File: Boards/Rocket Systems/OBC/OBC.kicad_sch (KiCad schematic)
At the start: 68 parts, among them IC1 NEO-M8Q-0, IC2 NSVT30010MXV6T1G, IC3 BC846BLT1G, J1 22027063, J2 5023520200, J3 SMARA_CONNECTOR, Q1 BC857CMB_315, U1 VLMKG3400-GS08, U2 LIS2MDLTR, U3 BMI323, U4 LSM6DSOTR, U5 LPS22DFTR, U6 BMP581

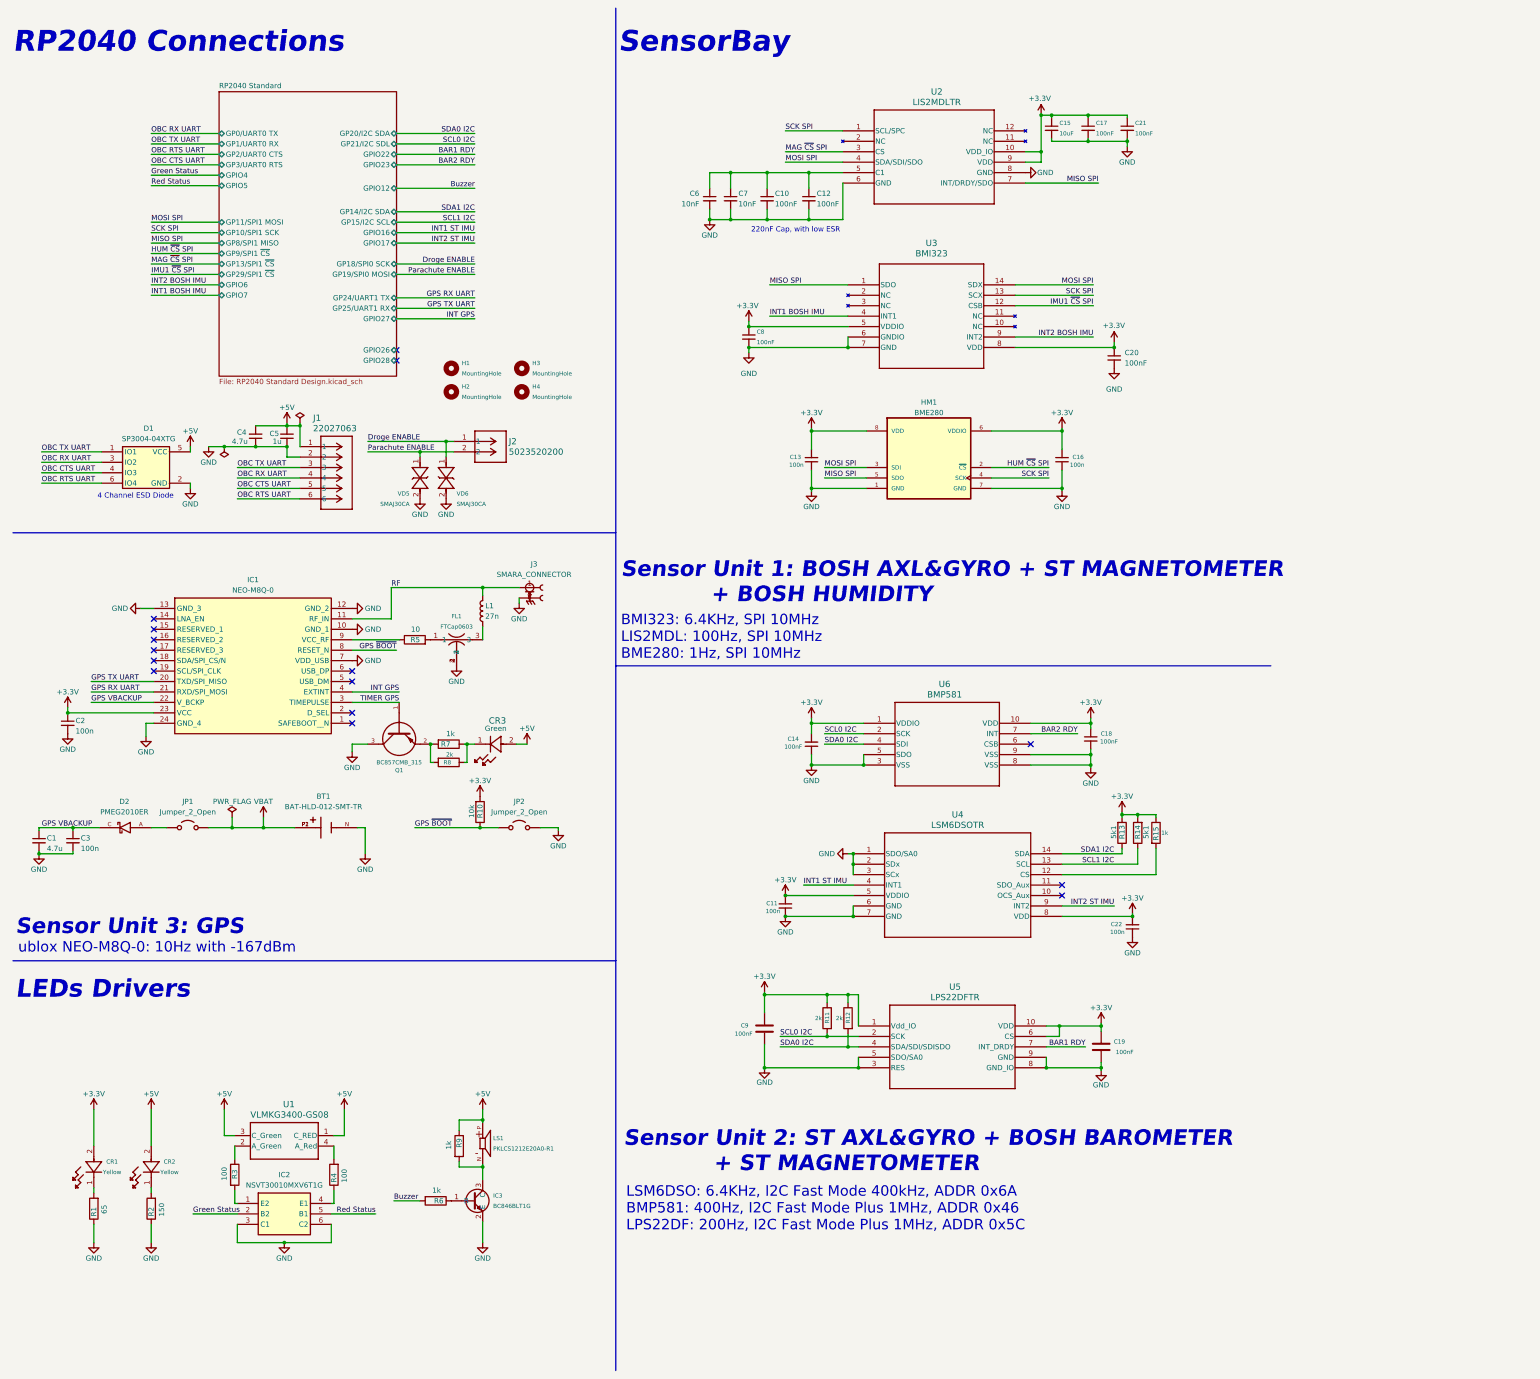
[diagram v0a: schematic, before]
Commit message: Repo rename and update
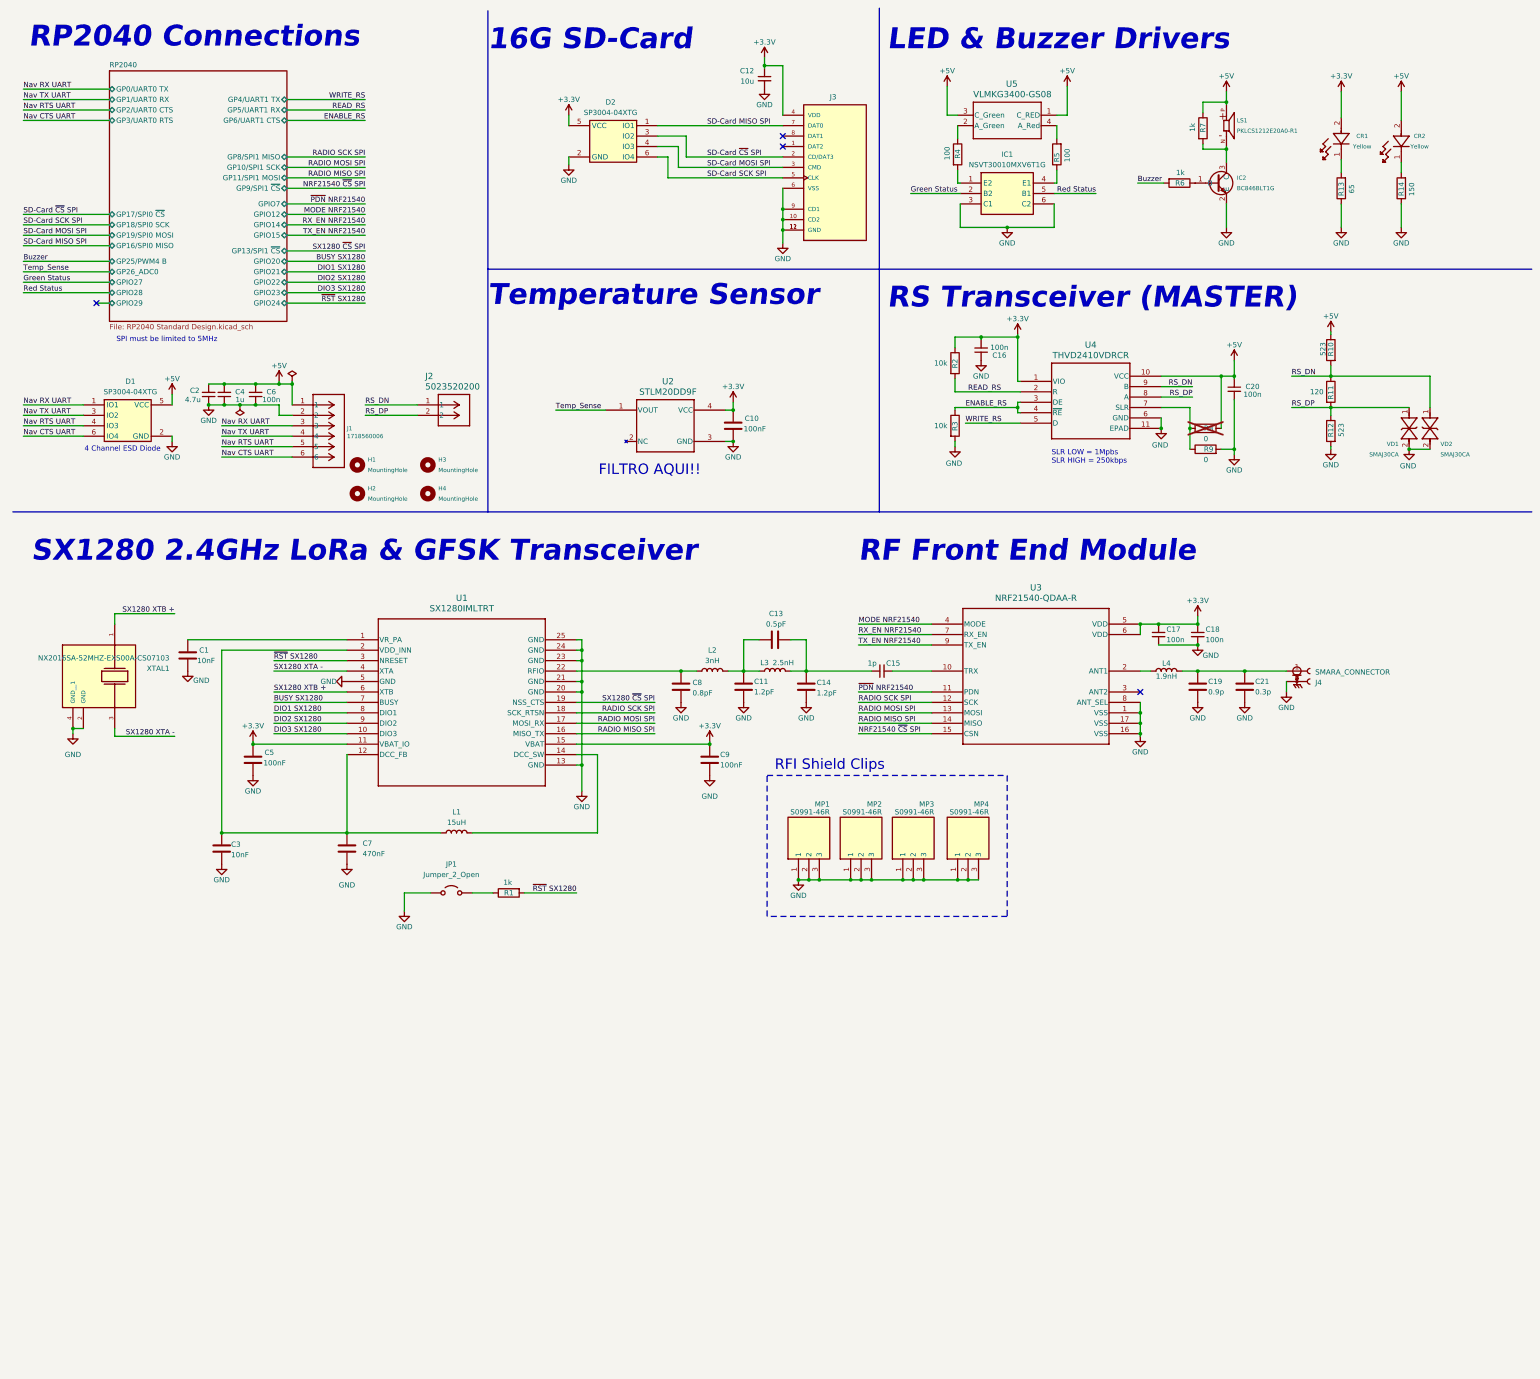
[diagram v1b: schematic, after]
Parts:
- removed BT1: BAT-HLD-012-SMT-TR, BAT_HLD_012:BAT_BAT-HLD-012-SMT-TR, symbol BAT-HLD-012-SMT-TR:BAT-HLD-012-SMT-TR
- removed C1: 4.7u, Capacitor-0402:Capacitor_0402, symbol Device:C_Small
- removed C10, C14, C21, C8: 100nF, Capacitor-0402:Capacitor_0402, symbol Device:C_Small
- removed C11, C13, C22, C3: 100n, Capacitor-0402:Capacitor_0402, symbol Device:C_Small
- removed C5: 1u, Capacitor-0402:Capacitor_0402, symbol Device:C_Small
- removed C7: 10nF, Capacitor-0402:Capacitor_0402, symbol Device:C_Small
- removed CR3: VLMC3100-GS08, LED-Green_VLMC3100-GS08:LED_PLCC_VSMB, symbol GreenLED__VLMC3100-GS08:VLMC3100-GS08
- removed D2: PMEG2010ER, Diode-Schottky_PMEG2010ER:SODFL3517X110N, symbol PMEG2010ER:PMEG2010ER
- removed FL1: FTCap0603, FTCap_0603:FTCap_0603, symbol FTCap0603:FTCap0603
- removed HM1: BME280, BME280:BME280, symbol BME280:BME280
- removed IC1: NEO-M8Q-0, NEO-M8Q-0:NEO-M8_UBL, symbol NEO-M8Q-0:NEO-M8Q-0
- removed IC2: NSVT30010MXV6T1G, 2 PNP:SOT-563_1P3X1P7_ONS, symbol NSVT30010MXV6T1G:NSVT30010MXV6T1G
- removed IC3: BC846BLT1G, BJT NPN:SOT96P237X111-3N, symbol BC846BLT1G:BC846BLT1G
- removed J1: 22027063, 6 Female Conn:CONN6X1_22027063_MOL, symbol 022027063:22027063
- removed J3: SMARA_CONNECTOR, Side Angle SMA:SMARACONNECTOR, symbol SMARA_CONNECTOR:SMARA_CONNECTOR
- removed JP2: Jumper_2_Open, Jumper:SolderJumper-2_P1.3mm_Open_RoundedPad1.0x1.5mm, symbol Jumper:Jumper_2_Open
- removed Q1: BC857CMB_315, PNP_BC857CMB_315:TRANS_PMZB550UNEYL, symbol BC857CMB_315:BC857CMB_315
- removed R15: 1k, Resistor-0402:RES_0402, symbol Device:R
- removed U1: VLMKG3400-GS08, VLMKG3400-GS08:SMT_00-GS08_VIS, symbol VLMKG3400-GS08:VLMKG3400-GS08
- removed U2: LIS2MDLTR, MAG LIS2MDLTR:LGA-12_2X2X1_STM, symbol MAG_LIS2MDLTR:LIS2MDLTR
- removed U3: BMI323, IMU BMI323:BMI323_BOS, symbol IMU_BMI323:BMI323
- removed U4: LSM6DSOTR, LSM6DSOTR:LGA-14L_2P5X3X0P86_STM, symbol LSM6DSOTR:LSM6DSOTR
- removed U5: LPS22DFTR, BARO LPS22DFTR:QFN_22DFTR_STM, symbol BARO_LPS22DFTR:LPS22DFTR
- removed U6: BMP581, BARO BMP581:QFN10_BMP581_BOS, symbol BARO_BMP581:BMP581
- removed VD5, VD6: SMAJ30CA, SMAJ30CA:SMASeries_LTF, symbol SMAJ30CA:SMAJ30CA
- added C1, C3: 10nF, Capacitor-0402:Capacitor_0402, symbol Device:C
- added C10, C5: 100nF, Capacitor-0402:Capacitor_0402, symbol Device:C
- added C11, C14: 1.2pF, Capacitor-0402:Capacitor_0402, symbol Device:C
- added C13: 0.5pF, Capacitor-0402:Capacitor_0402, symbol Device:C
- added C21: 0.3p, Capacitor-0402:Capacitor_0402, symbol Device:C
- added C7: 470nF, Capacitor-0402:Capacitor_0402, symbol Device:C
- added C8: 0.8pF, Capacitor-0402:Capacitor_0402, symbol Device:C
- added D2: SP3004-04XTG, TVS-SP3004:SOT563_LTF, symbol SP3004-04XTG:SP3004-04XTG
- added IC1: NSVT30010MXV6T1G, 2 PNP:SOT-563_1P3X1P7_ONS, symbol NSVT30010MXV6T1G:NSVT30010MXV6T1G
- added IC2: BC846BLT1G, BJT NPN:SOT96P237X111-3N, symbol BC846BLT1G:BC846BLT1G
- added J1: 1718560006, 6 Male Conn:CONN06_1718560006_MOL, symbol 1718560006:1718560006
- added J3: MEM2061-01-188-00-A_REVA, SD-CARD_MEM2061-01-188-00-A:GCT_MEM2061-01-188-00-A_REVA, symbol MEM2061-01-188-00-A_REVA:MEM2061-01-188-00-A_REVA
- added J4: SMARA_CONNECTOR, Side Angle SMA:SMARACONNECTOR, symbol SMARA_CONNECTOR:SMARA_CONNECTOR
- added L2: 3nH, Inductor-0402:Inductor_0402, symbol Device:L
- added L3: 2.5nH, Inductor-0402:Inductor_0402, symbol Device:L
- added L4: 1.9nH, Inductor-0201:Inductor_0201, symbol Device:L
- added MP1, MP2, MP3, MP4: S0991-46R, S0991-46R:S099146R, symbol S0991-46R:S0991-46R
- added U1: SX1280IMLTRT, SX1280:QFN24_4X4_SEM, symbol SX1280:SX1280IMLTRT
- added U2: STLM20DD9F, STLM20DD9F:UDFN-4L_STM, symbol STLM20DD9F:STLM20DD9F
- added U3: NRF21540-QDAA-R, RF FEM:QFN16_4X4_NOR, symbol NRF21540-QDAA-R:NRF21540-QDAA-R
- added U4: THVD2410VDRCR, THVD2410VDRCR:VSON10_DRC_TEX, symbol THVD2410VDRCR:THVD2410VDRCR
- added U5: VLMKG3400-GS08, VLMKG3400-GS08:SMT_00-GS08_VIS, symbol VLMKG3400-GS08:VLMKG3400-GS08
- added VD1, VD2: SMAJ30CA, SMAJ30CA:SMASeries_LTF, symbol SMAJ30CA:SMAJ30CA
- added XTAL1: NX2016SA-52MHZ-EXS00A-CS07103, NX2016SA_52MHZ:OSCCC200X160X50N, symbol NX2016SA-52MHZ-EXS00A-CS07103:NX2016SA-52MHZ-EXS00A-CS07103
- C12: value 100nF -> 10u; footprint Capacitor-0402:Capacitor_0402 -> Capacitor-0805:Capacitor_0805
- C15: value 10uF -> 1p; footprint Capacitor-0805:Capacitor_0805 -> Capacitor-0402:Capacitor_0402
- C17, C18, C20: value 100nF -> 100n
- C19: value 100nF -> 0.9p
- C2: value 100n -> 4.7u
- C4: value 4.7u -> 1u
- C6: value 10nF -> 100n
- L1: value 27n -> 15uH; footprint Inductor-0402:Inductor_0402 -> Inductor-0805:Inductor_0805
- R1: value 65 -> 1k
- R10: value 10k -> 523
- R11: value 2k -> 120; footprint Resistor-0402:RES_0402 -> Resistor-0603:RES_0603
- R12: value 2k -> 523
- R13: value 5k1 -> 65
- R14: value 5k1 -> 150
- R2: value 150 -> 10k
- R3: value 100 -> 10k
- R5: value 10 -> 100
- R8: value 2k -> 0; now not fitted; now left out of the parts list
- R9: value 1k -> 0
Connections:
- net GPS ~{BOOT} is gone; now on net +5V: R10.1
- net SCL0 I2C is gone; now on net RS_DP: R11.2
- net SCL1 I2C is gone; now on net GND: R14.1
- net SDA0 I2C is gone; now on net GND: R12.2
- net SDA1 I2C is gone; now on net GND: R13.1
- net +3.3V: now also C12.1, C9.1, R2.1, C10.1, C5.1, D2.5 (VCC), J3.4 (VDD), U1.11 (VBAT_IO), U1.15 (VBAT), U2.4 (VCC), U3.5 (VDD), U3.6 (VDD), U4.1 (VIO); no longer C15.1, C19.2, C2.1, C20.1, C9.2, R10.2, R11.1, R12.1, R13.2, R14.2
- net +5V: now also C2.2, C20.1, C6.2, R7.1, R8.2, J1.1, U4.10 (VCC), U5.1 (C_RED), U5.3 (C_Green); no longer R9.1
- net GND: now also C19.2, C2.1, C6.1, C9.2, JP1.1 (A), R3.2, R9.2, C1.2, C10.2, C11.2, C14.2, C21.2, C3.2, C5.2, C7.2, C8.2, D2.2 (GND), IC1.3 (C1), IC1.6 (C2), IC2.2 (E), J1.2, J3.10 (CD2), J3.11 (GND), J3.12 (GND), J3.6 (VSS), J3.9 (CD1), J4.2, J4.3, J4.4, J4.5, MP1.1, MP1.2, MP1.3, MP2.1, MP2.2, MP2.3, MP3.1, MP3.2, MP3.3, MP4.1, MP4.2, MP4.3, U1.13 (GND), U1.20 (GND), U1.21 (GND), U1.23 (GND), U1.24 (GND), U1.25 (GND), U1.5 (GND), U2.3 (GND), U3.1 (VSS), U3.16 (VSS), U3.17 (VSS), U3.8 (ANT_SEL), U4.11 (EPAD), U4.6 (GND), VD1.2, VD2.2, XTAL1.2 (GND), XTAL1.4 (GND__1); no longer C15.2, C19.1, C2.2, C6.2, C9.1, R1.1, R2.1
- net Green Status: now also IC1.2 (B2)
- net Red Status: now also IC1.5 (B1)
- net ENABLE_RS: now reaches R3.1
- net ENABLE_RS: now also U4.3 (DE), U4.4 (~{RE})
- net at R4.2: now also IC1.1 (E2)
- net at LS1.N: now also R7.2, IC2.3 (C); no longer R9.2
- net at R6.1: now also IC2.1 (B)
- net at CR1.1: now also R13.2; no longer R1.2
- net at R8.1: now also R9.1, U4.7 (SLR); no longer R7.1
- net at R5.2: now also U5.4 (A_Red)
- net at L1.1: now also C3.1, C7.1, U1.12 (DCC_FB), U1.2 (VDD_INN)
- net at R4.1: now also U5.2 (A_Green)
- net at R5.1: now also IC1.4 (E1)
- net at CR2.1: now also R14.2; no longer R2.2
- net Droge ENABLE renamed RS_DN
- net RS_DN: now also R10.2, R11.1, U4.9 (B), VD2.1
- net OBC CTS UART renamed Nav RTS UART
- net Nav RTS UART: now also J1.5
- net OBC RTS UART renamed Nav CTS UART
- net Nav CTS UART: now also J1.6
- net OBC RX UART renamed Nav TX UART
- net Nav TX UART: now also J1.4
- net OBC TX UART renamed Nav RX UART
- net Nav RX UART: now also J1.3
- net Parachute ENABLE renamed RS_DP
- net RS_DP: now also R12.1, U4.8 (A), VD1.1
- net RF: no longer names the net of L1.2
- net RF: now also U1.14 (DCC_SW)
- net VBAT: no longer names the net of JP1.2 (B)
- net VBAT: now also R1.1
- new net: C1.1, U1.1 (VR_PA)
- new net: C8.1, L2.1, U1.22 (RFIO)
- new net: C11.1, C13.2, L2.2, L3.1
- new net: C13.1, C14.1, C15.1, L3.2
- new net: C19.1, C21.1, J4.1, L4.2
- new net: C15.2, U3.10 (TRX)
- new net: L4.1, U3.2 (ANT1)
- new net BUSY SX1280: U1.7 (BUSY)
- new net DIO1 SX1280: U1.8 (DIO1)
- new net DIO2 SX1280: U1.9 (DIO2)
- new net DIO3 SX1280: U1.10 (DIO3)
- new net MODE NRF21540: U3.4 (MODE)
- new net NRF21540 ~{CS} SPI: U3.15 (CSN)
- new net RADIO MISO SPI: U1.16 (MISO_TX), U3.14 (MISO)
- new net RADIO MOSI SPI: U1.17 (MOSI_RX), U3.13 (MOSI)
- new net RADIO SCK SPI: U1.18 (SCK_RTSN), U3.12 (SCK)
- new net READ_RS: R2.2, U4.2 (R)
- new net RX_EN NRF21540: U3.7 (RX_EN)
- new net SD-Card  ~{CS} SPI: D2.3 (IO2), J3.2 (CD/DAT3)
- new net SD-Card MISO SPI: D2.1 (IO1), J3.7 (DAT0)
- new net SD-Card MOSI SPI: D2.4 (IO3), J3.3 (CMD)
- new net SD-Card SCK SPI: D2.6 (IO4), J3.5 (CLK)
- new net SX1280 XTA -: U1.4 (XTA), XTAL1.3
- new net SX1280 XTB +: U1.6 (XTB), XTAL1.1
- new net SX1280 ~{CS} SPI: U1.19 (NSS_CTS)
- new net TX_EN NRF21540: U3.9 (TX_EN)
- new net Temp_Sense: U2.1 (VOUT)
- new net WRITE_RS: U4.5 (D)
- new net ~{PDN} NRF21540: U3.11 (PDN)
- new net ~{RST} SX1280: R1.2, U1.3 (NRESET)
- no-connect marks 15 -> 4
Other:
- removed sheet RP2040 Standard
- added sheet RP2040 (RP2040 Standard Design.kicad_sch)
- note added: "16G SD-Card"
- note added: "FILTRO AQUI!!"
- note added: "LED & Buzzer Drivers"
- note added: "RF Front End Module"
- note added: "RFI Shield Clips"
- note added: "RS Transceiver (MASTER)"
- note added: "SLR LOW = 1Mpbs SLR HIGH = 250kbps"
- note added: "SPI must be limited to 5MHz"
- note added: "SX1280 2.4GHz LoRa & GFSK Transceiver"
- note added: "Temperature Sensor"
- note removed: "220nF Cap, with low ESR"
- note removed: "BMI323: 6.4KHz, SPI 10MHz LIS2MDL: 100Hz, SPI 10MHz BME280: 1Hz, SPI 10MHz"
- note removed: "LEDs Drivers"
- note removed: "LSM6DSO: 6.4KHz, I2C Fast Mode 400kHz, ADDR 0x6A BMP581: 400Hz, I2C Fast Mode Plus 1MHz, ADDR 0x46 LPS22DF: 200Hz, I2C Fast Mode Plus 1MHz, ADDR 0x5C"
- note removed: "Sensor Unit 1: BOSH AXL&GYRO + ST MAGNETOMETER + BOSH HUMIDITY"
- note removed: "Sensor Unit 2: ST AXL&GYRO + BOSH BAROMETER + ST MAGNETOMETER"
- note removed: "Sensor Unit 3: GPS"
- note removed: "SensorBay"
- note removed: "ublox NEO-M8Q-0: 10Hz with -167dBm"
- title: Navigator -> On Board Computer
- moved on the sheet: H1, H2, H3, H4, LS1
